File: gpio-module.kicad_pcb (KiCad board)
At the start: 4 copper layers, 100 x 100 mm, 196 parts, among them J10 Molex_Micro-Fit_3.0 2x2, J11 Molex_Micro-Fit_3.0 2x2, J200 09031967921, J8 Molex_Micro-Fit_3.0 2x2, J800 USB_C_Receptacle_USB2.0_16P, J9 Molex_Micro-Fit_3.0 2x2, Q401 AO3400A, Q402 AO3400A, Q403 AO3400A, Q405 AO3400A, Q406 AO3400A, Q407 AO3400A, Q700 MMST3904, U100 W25Q128, U300 TPS563200, U301 TPS563200, U302 CH334P, U401 TPD2E2U06DCK, U402 TPD2E2U06DCK, U403 STM32H562VGTx, U500 TJA1044GTK_3Z, U600 TJA1044GTK_3Z, U700 STM32F103CBTx, U801 FSUSB42UMX, X300 Q13FC1350000400, Y400 ASE-xxxMHz, Y700 Crystal_GND24, Y900 Crystal_GND24

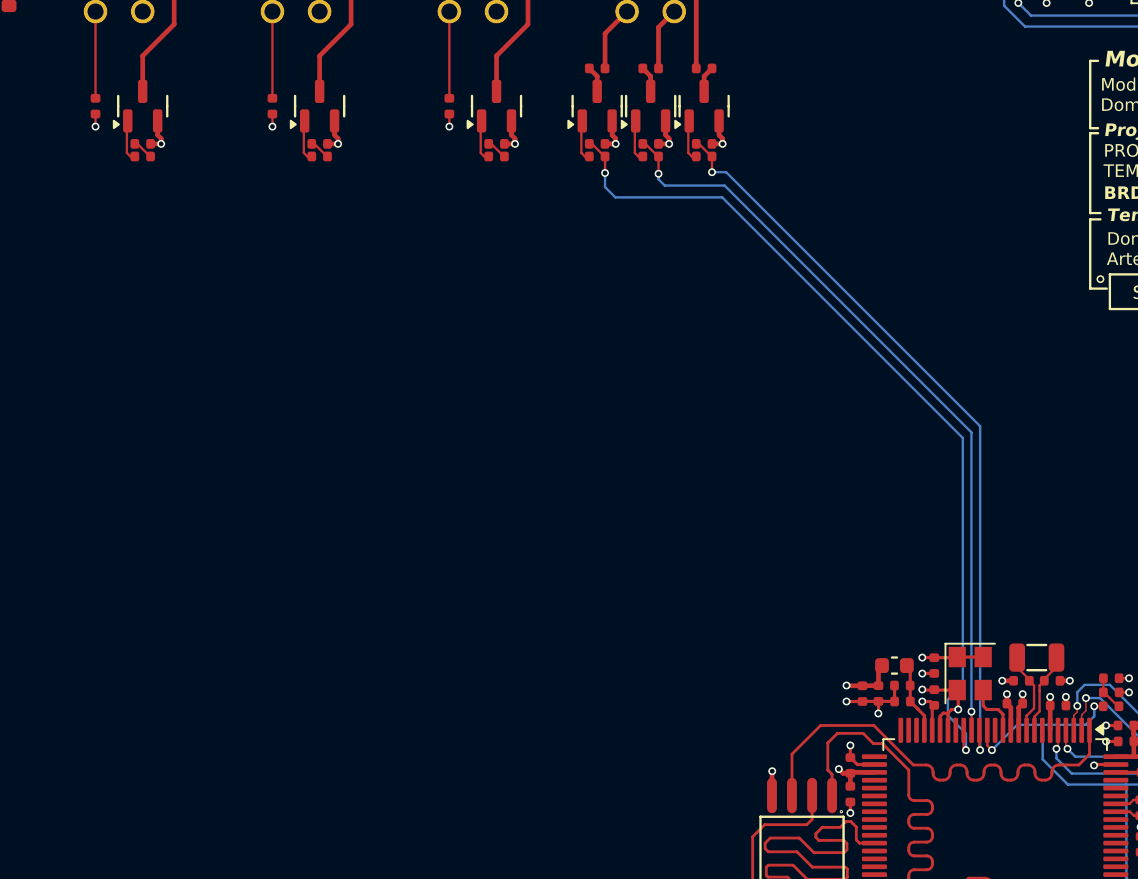
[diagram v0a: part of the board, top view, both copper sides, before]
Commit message: [#1] Connect all GPIO connectors to MCU
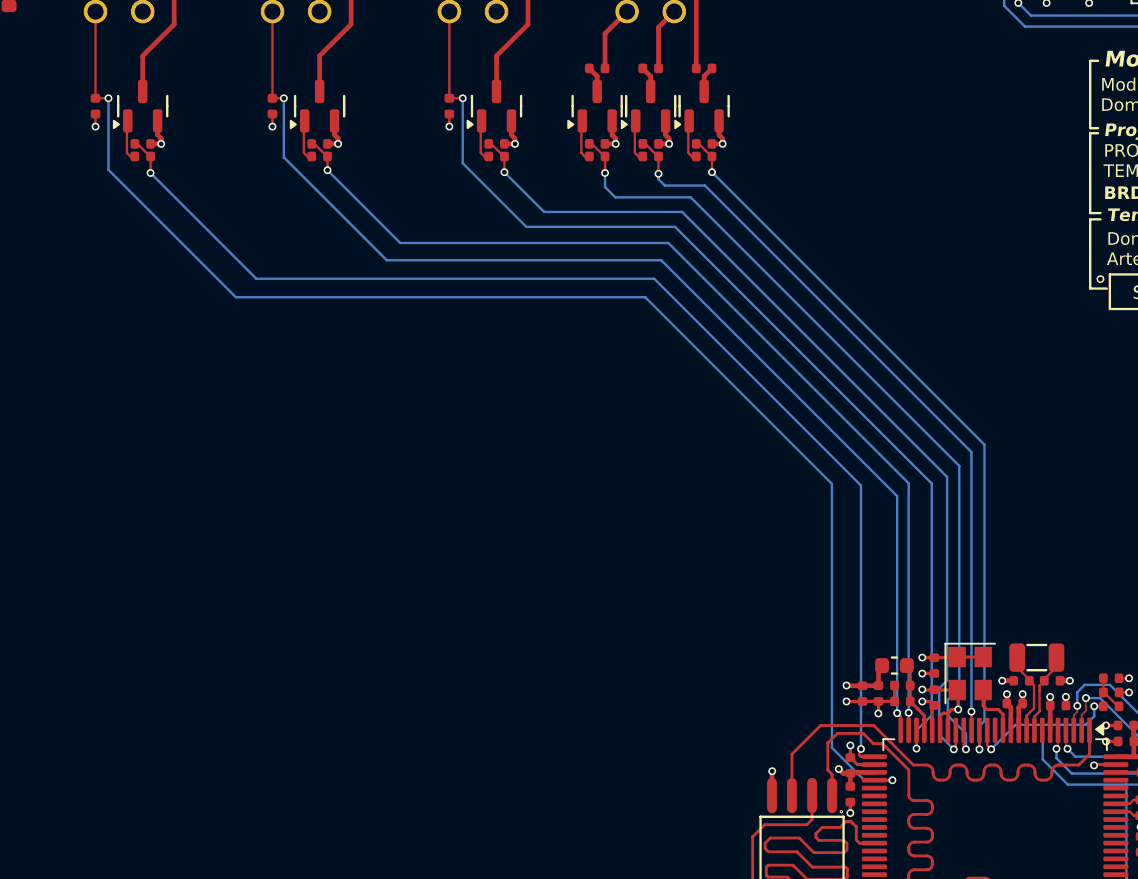
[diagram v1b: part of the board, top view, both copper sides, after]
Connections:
- net /GPIO connector/MOSFET power stage/output renamed /GPIO connector 0/MOSFET power stage/output
- net /GPIO connector1/MOSFET power stage/output renamed /GPIO connector 1/MOSFET power stage/output
- net /GPIO connector2/MOSFET power stage/output renamed /GPIO connector 2/MOSFET power stage/output
- J10 pad 3: /GPIO connector1/input -> /GPIO connector 1/input
- J11 pad 3: /GPIO connector2/input -> /GPIO connector 2/input
- J9 pad 3: /GPIO connector/input -> /GPIO connector 0/input
- R422 pad 1: /GPIO connector/input -> /GPIO connector 0/input
- R423 pad 1: /GPIO connector/output -> /GPIO connector 0/output
- R424 pad 1: /GPIO connector1/input -> /GPIO connector 1/input
- R425 pad 1: /GPIO connector1/output -> /GPIO connector 1/output
- R426 pad 1: /GPIO connector/output -> /GPIO connector 0/output
- R427 pad 1: /GPIO connector1/output -> /GPIO connector 1/output
- R428 pad 1: /GPIO connector2/input -> /GPIO connector 2/input
- R429 pad 1: /GPIO connector2/output -> /GPIO connector 2/output
- R430 pad 1: /GPIO connector2/output -> /GPIO connector 2/output
- U403 pad 18: unconnected-(U403-PC3-Pad18) -> /GPIO connector 0/output
- U403 pad 23: unconnected-(U403-PA0-Pad23) -> /GPIO connector 0/input
- U403 pad 24: unconnected-(U403-PA1-Pad24) -> /GPIO connector 1/output
- U403 pad 25: unconnected-(U403-PA2-Pad25) -> /GPIO connector 1/input
- U403 pad 26: unconnected-(U403-PA3-Pad26) -> /GPIO connector 2/output
- U403 pad 29: unconnected-(U403-PA4-Pad29) -> /GPIO connector 2/input
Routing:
- net /GPIO connector 2/input: track 0.00 -> 87.8 mm, vias 0 -> 2
- net /GPIO connector 2/output: track 0.00 -> 74.0 mm, vias 0 -> 2
- net /GPIO connector 1/input: track 0.00 -> 72.9 mm, vias 0 -> 2
- net /GPIO connector 0/input: track 0.00 -> 67.2 mm, vias 0 -> 2
- net /GPIO connector 1/output: track 0.00 -> 63.1 mm, vias 0 -> 2
- net /GPIO connector 0/output: track 0.00 -> 57.7 mm, vias 0 -> 2
- net /GPIO connector2/input: track 5.52 -> 0.00 mm
- net /GPIO connector1/input: track 5.52 -> 0.00 mm
- net /GPIO connector/input: track 5.52 -> 0.00 mm
- net /MCU/EXT_LED_G: track 54.7 -> 53.2 mm
- net /GPIO connector2/output: track 1.33 -> 0.00 mm
- net /GPIO connector1/output: track 1.33 -> 0.00 mm
- net /GPIO connector/output: track 1.33 -> 0.00 mm
- net /MCU/EXT_LED_R: track 48.3 -> 47.6 mm

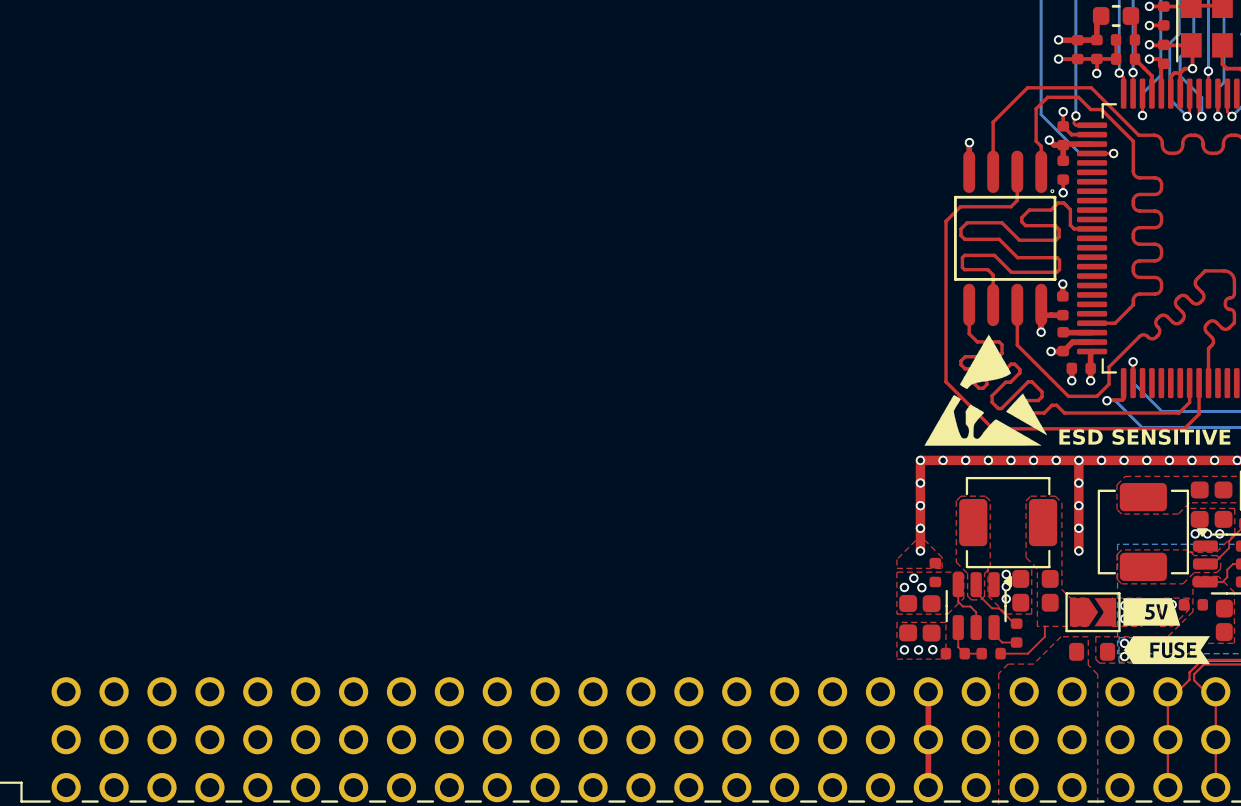
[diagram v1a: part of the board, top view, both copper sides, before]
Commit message: [#1] Connect GPIOR to MCU
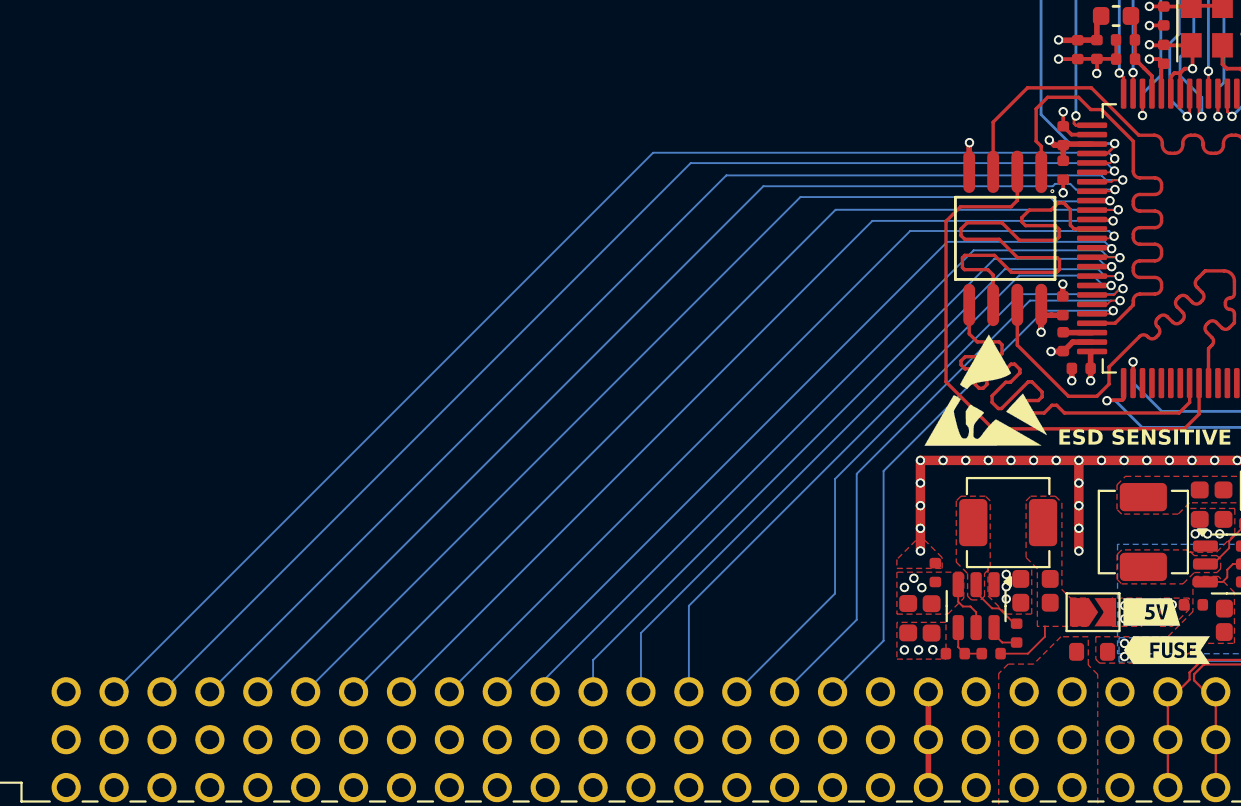
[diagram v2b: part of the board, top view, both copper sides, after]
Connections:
- U403 pad 30: unconnected-(U403-PA5-Pad30) -> /Backplane/GPIOR15
- U403 pad 31: unconnected-(U403-PA6-Pad31) -> /Backplane/GPIOR14
- U403 pad 32: unconnected-(U403-PA7-Pad32) -> /Backplane/GPIOR13
- U403 pad 33: unconnected-(U403-PC4-Pad33) -> /Backplane/GPIOR12
- U403 pad 34: unconnected-(U403-PC5-Pad34) -> /Backplane/GPIOR11
- U403 pad 35: unconnected-(U403-PB0-Pad35) -> /Backplane/GPIOR10
- U403 pad 36: unconnected-(U403-PB1-Pad36) -> /Backplane/GPIOR9
- U403 pad 38: unconnected-(U403-PE7-Pad38) -> /Backplane/GPIOR8
- U403 pad 39: unconnected-(U403-PE8-Pad39) -> /Backplane/GPIOR7
- U403 pad 40: unconnected-(U403-PE9-Pad40) -> /Backplane/GPIOR6
- U403 pad 41: unconnected-(U403-PE10-Pad41) -> /Backplane/GPIOR5
- U403 pad 42: unconnected-(U403-PE11-Pad42) -> /Backplane/GPIOR4
- U403 pad 43: unconnected-(U403-PE12-Pad43) -> /Backplane/GPIOR3
- U403 pad 44: unconnected-(U403-PE13-Pad44) -> /Backplane/GPIOR2
- U403 pad 45: unconnected-(U403-PE14-Pad45) -> /Backplane/GPIOR1
- U403 pad 46: unconnected-(U403-PE15-Pad46) -> /Backplane/GPIOR0
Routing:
- net /Backplane/GPIOR15: track 0.00 -> 66.3 mm, vias 0 -> 1
- net /Backplane/GPIOR14: track 0.00 -> 63.5 mm, vias 0 -> 1
- net /Backplane/GPIOR13: track 0.00 -> 61.5 mm, vias 0 -> 1
- net /Backplane/GPIOR12: track 0.00 -> 58.0 mm, vias 0 -> 1
- net /Backplane/GPIOR11: track 0.00 -> 54.6 mm, vias 0 -> 1
- net /Backplane/GPIOR10: track 0.00 -> 52.5 mm, vias 0 -> 1
- net /Backplane/GPIOR9: track 0.00 -> 49.2 mm, vias 0 -> 1
- net /Backplane/GPIOR8: track 0.00 -> 46.7 mm, vias 0 -> 1
- net /Backplane/GPIOR7: track 0.00 -> 43.7 mm, vias 0 -> 1
- net /Backplane/GPIOR6: track 0.00 -> 42.3 mm, vias 0 -> 1
- net /Backplane/GPIOR5: track 0.00 -> 39.2 mm, vias 0 -> 1
- net /Backplane/GPIOR4: track 0.00 -> 38.1 mm, vias 0 -> 1
- net /Backplane/GPIOR3: track 0.00 -> 35.4 mm, vias 0 -> 1
- net /Backplane/GPIOR2: track 0.00 -> 34.7 mm, vias 0 -> 1
- net /Backplane/GPIOR1: track 0.00 -> 32.5 mm, vias 0 -> 1
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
